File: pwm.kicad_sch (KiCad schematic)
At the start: 25 parts, among them IC1 UCC28180D, Q4 T2N7002AK, U16 MCP6562, U17 74LVC1G02, U18 74LVC1G02, U3 UCC21520DW, U9 CD4053B

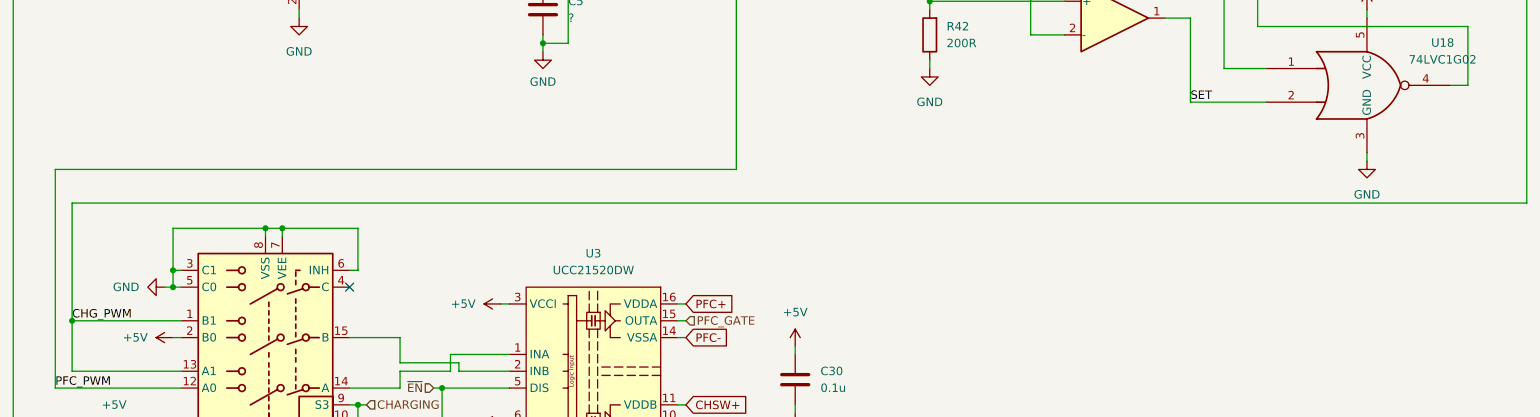
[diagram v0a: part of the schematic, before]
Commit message: final touches?
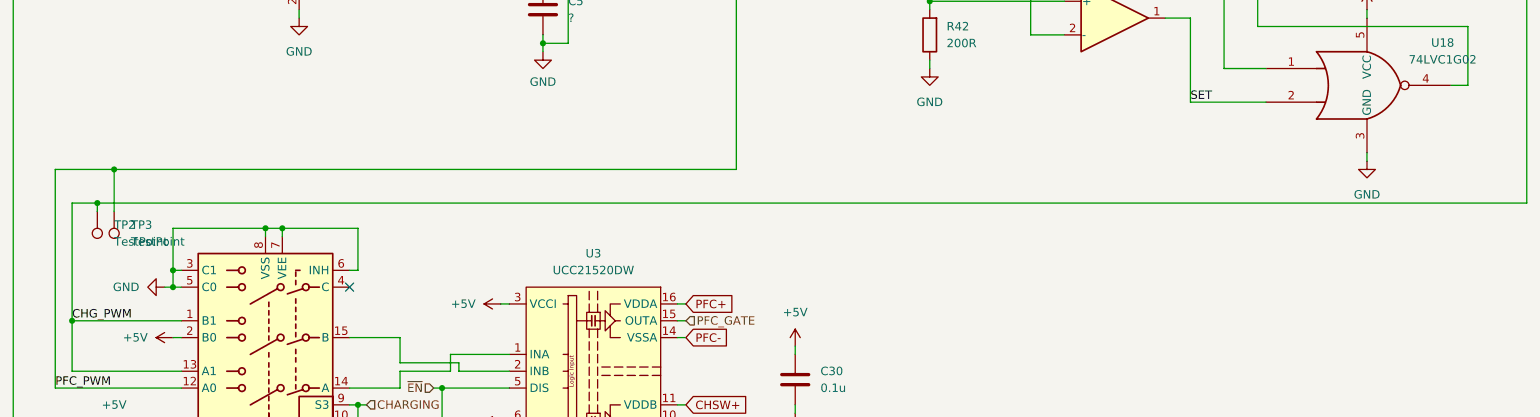
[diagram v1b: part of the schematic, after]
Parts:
- added TP2, TP3: TestPoint, TestPoint:TestPoint_Pad_1.0x1.0mm, symbol Connector:TestPoint
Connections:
- net CHG_PWM: now also TP2.1
- net PFC_PWM: now also TP3.1
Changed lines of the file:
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@@
 	)
 	(junction
+		(at 60.96 107.95)
+		(diameter 0)
+		(color 0 0 0 0)
+	)
+	(junction
 		(at 88.9 111.76)
 		(diameter 0)
@@
 	)
 	(junction
+		(at 63.5 102.87)
+		(diameter 0)
+		(color 0 0 0 0)
+	)
+	(junction
 		(at 170.18 31.75)
 		(diameter 0)
@@
 	(wire
 		(pts
+			(xy 60.96 107.95) (xy 276.86 107.95)
+		)
+		(stroke
+			(width 0)
+			(type default)
+		)
+	)
+	(wire
+		(pts
 			(xy 86.36 111.76) (xy 88.9 111.76)
 		)
@@
 	(wire
 		(pts
-			(xy 157.48 102.87) (xy 54.61 102.87)
+			(xy 157.48 102.87) (xy 63.5 102.87)
 		)
 		(stroke
@@
 	(wire
 		(pts
-			(xy 57.15 107.95) (xy 276.86 107.95)
+			(xy 57.15 107.95) (xy 60.96 107.95)
 		)
 		(stroke
@@
 	(wire
 		(pts
+			(xy 60.96 107.95) (xy 60.96 109.22)
+		)
+		(stroke
+			(width 0)
+			(type default)
+		)
+	)
+	(wire
+		(pts
 			(xy 186.69 66.04) (xy 186.69 67.31)
 		)
@@
 	(wire
 		(pts
+			(xy 63.5 102.87) (xy 63.5 109.22)
+		)
+		(stroke
+			(width 0)
+			(type default)
+		)
+	)
+	(wire
+		(pts
 			(xy 106.68 128.27) (xy 106.68 132.08)
 		)
@@
 	(wire
 		(pts
+			(xy 63.5 102.87) (xy 54.61 102.87)
+		)
+		(stroke
+			(width 0)
+			(type default)
+		)
+	)
+	(wire
+		(pts
 			(xy 222.25 64.77) (xy 226.06 64.77)
 		)
@@
 	)
 	(symbol
+		(lib_id "Connector:TestPoint")
+		(at 60.96 109.22 180)
+		(unit 1)
+		(body_style 1)
+		(exclude_from_sim no)
+		(in_bom yes)
+		(on_board yes)
+		(in_pos_files yes)
+		(dnp no)
+		(fields_autoplaced yes)
+		(property "Reference" "TP2"
+			(at 63.5 111.2519 0)
+			(show_name no)
+			(do_not_autoplace no)
+			(effects
+				(font
+					(size 1.27 1.27)
+				)
+				(justify right)
+			)
+		)
+		(property "Value" "TestPoint"
+			(at 63.5 113.7919 0)
+			(show_name no)
+			(do_not_autoplace no)
+			(effects
+				(font
+					(size 1.27 1.27)
+				)
+				(justify right)
+			)
+		)
+		(property "Footprint" "TestPoint:TestPoint_Pad_1.0x1.0mm"
+			(at 55.88 109.22 0)
+			(hide yes)
+			(show_name no)
+			(do_not_autoplace no)
+			(effects
+				(font
+					(size 1.27 1.27)
+				)
+			)
+		)
+		(property "Datasheet" ""
+			(at 55.88 109.22 0)
+			(hide yes)
+			(show_name no)
+			(do_not_autoplace no)
+			(effects
+				(font
+					(size 1.27 1.27)
+				)
+			)
+		)
+		(property "Description" "test point"
+			(at 60.96 109.22 0)
+			(hide yes)
+			(show_name no)
+			(do_not_autoplace no)
+			(effects
+				(font
+					(size 1.27 1.27)
+				)
+			)
+		)
+		(pin "1"
+		)
+		(instances
+			(project "PFC"
+				(path "/9a4457e8-cc73-4b75-ac20-82cc64952613/9983a37e-d578-4b38-a394-f60aff5d4a98"
+					(reference "TP2")
+					(unit 1)
+				)
+			)
+		)
+	)
+	(symbol
 		(lib_id "power:GND")
 		(at 186.69 87.63 0)
@@
 					(unit 1)
 				)
+			)
+		)
+	)
+	(symbol
+		(lib_id "Connector:TestPoint")
+		(at 63.5 109.22 180)
+		(unit 1)
+		(body_style 1)
+		(exclude_from_sim no)
+		(in_bom yes)
+		(on_board yes)
+		(in_pos_files yes)
+		(dnp no)
+		(fields_autoplaced yes)
+		(property "Reference" "TP3"
+			(at 66.04 111.2519 0)
+			(show_name no)
+			(do_not_autoplace no)
+			(effects
+				(font
+					(size 1.27 1.27)
+				)
+				(justify right)
+			)
+		)
+		(property "Value" "TestPoint"
+			(at 66.04 113.7919 0)
+			(show_name no)
+			(do_not_autoplace no)
+			(effects
+				(font
+					(size 1.27 1.27)
+				)
+				(justify right)
+			)
+		)
+		(property "Footprint" "TestPoint:TestPoint_Pad_1.0x1.0mm"
+			(at 58.42 109.22 0)
+			(hide yes)
+			(show_name no)
+			(do_not_autoplace no)
+			(effects
+				(font
+					(size 1.27 1.27)
+				)
+			)
+		)
+		(property "Datasheet" ""
+			(at 58.42 109.22 0)
+			(hide yes)
+			(show_name no)
+			(do_not_autoplace no)
+			(effects
+				(font
+					(size 1.27 1.27)
+				)
+			)
+		)
+		(property "Description" "test point"
+			(at 63.5 109.22 0)
+			(hide yes)
+			(show_name no)
+			(do_not_autoplace no)
+			(effects
+				(font
+					(size 1.27 1.27)
+				)
+			)
+		)
+		(pin "1"
+		)
+		(instances
+			(project "PFC"
+				(path "/9a4457e8-cc73-4b75-ac20-82cc64952613/9983a37e-d578-4b38-a394-f60aff5d4a98"
+					(reference "TP3")
+					(unit 1)
+				)
